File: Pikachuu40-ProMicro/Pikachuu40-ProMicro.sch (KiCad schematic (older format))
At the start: 93 parts, among them K1 KEYSW, K10 KEYSW, K11 KEYSW, K12 KEYSW, K13 KEYSW, K14 KEYSW, K15 KEYSW, K16 KEYSW, K17 KEYSW, K18 KEYSW, K19 KEYSW, K2 KEYSW, K20 KEYSW, K21 KEYSW, K22 KEYSW, K23 KEYSW, K24 KEYSW, K25 KEYSW, K26 KEYSW, K27 KEYSW, K28 KEYSW, K29 KEYSW, K3 KEYSW, K30 KEYSW, K31 KEYSW, K32 KEYSW, K33 KEYSW, K34 KEYSW, K35 KEYSW, K36 KEYSW, K37 KEYSW, K38 KEYSW, K39 KEYSW, K4 KEYSW, K40 KEYSW, K41 KEYSW, K42 KEYSW, K43 KEYSW, K44 KEYSW, K45 KEYSW, K5 KEYSW, K6 KEYSW, K7 KEYSW, K8 KEYSW, K9 KEYSW, U1 ProMicro

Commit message: Schematic done again
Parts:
- K1, K10, K11, K12, K13, K14, K15, K16, K17, K18, K19, K2, K20, K21, K22, K23, K24, K25, K26, K27, K28, K29, K3, K30, K31, K32, K33, K34, K35, K36, K37, K38, K39, K4, K40, K41, K42, K43, K44, K45, K5, K6, K7, K8, K9, K?1: footprint Keebio-Parts:MX_LED -> Button_Switch_Keyboard:SW_Cherry_MX_1.00u_PCB

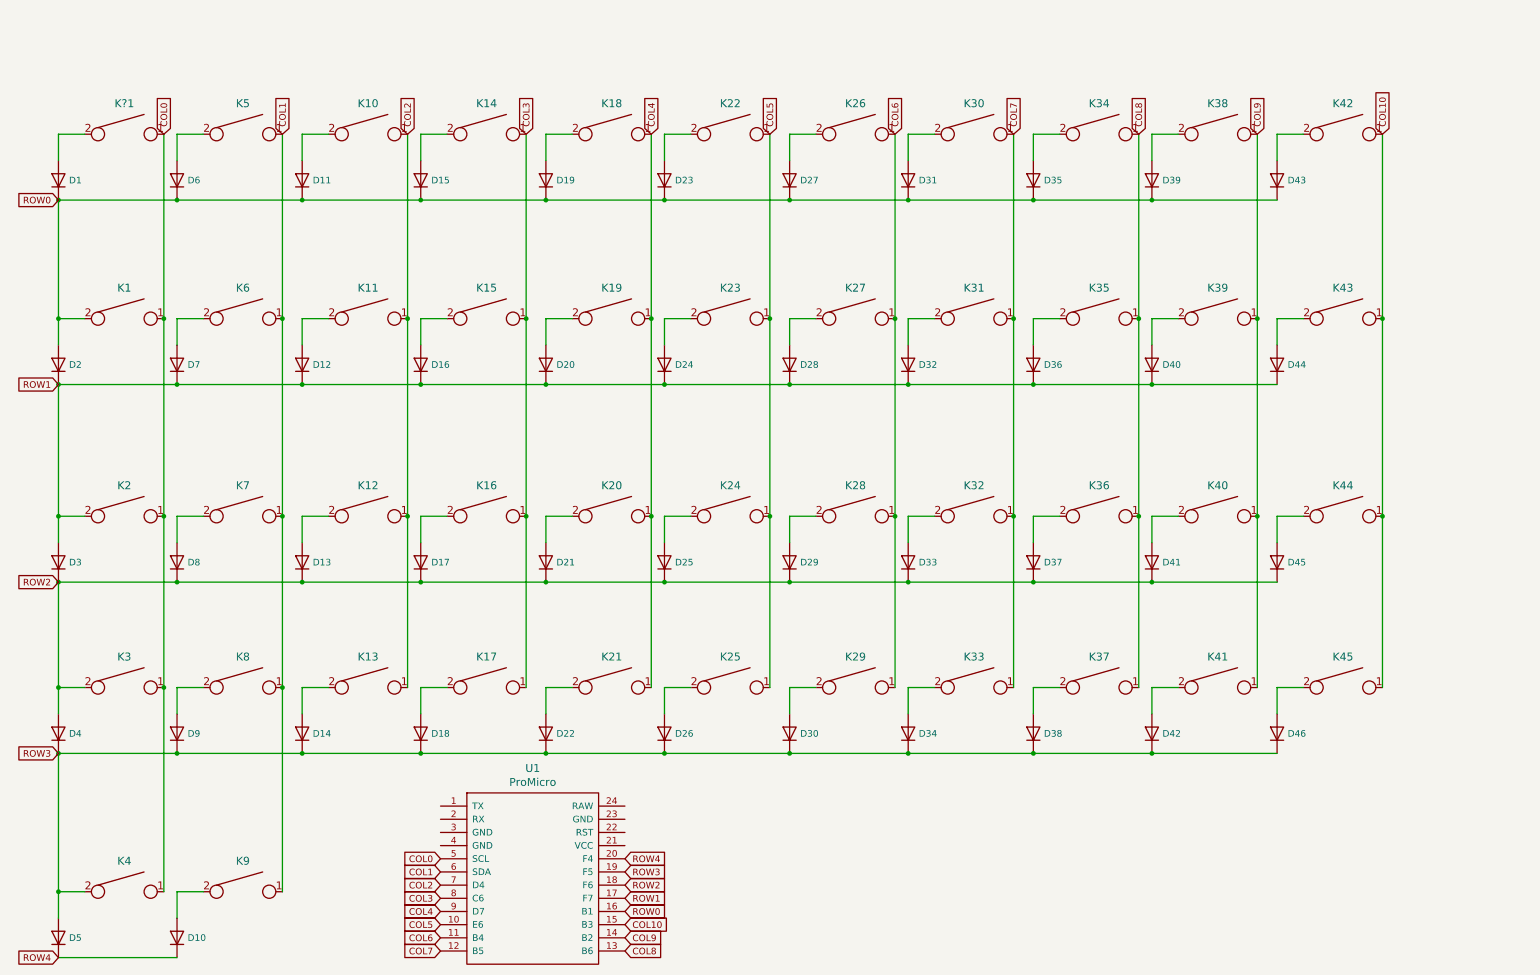
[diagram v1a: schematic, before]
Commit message: Rough Routing Done
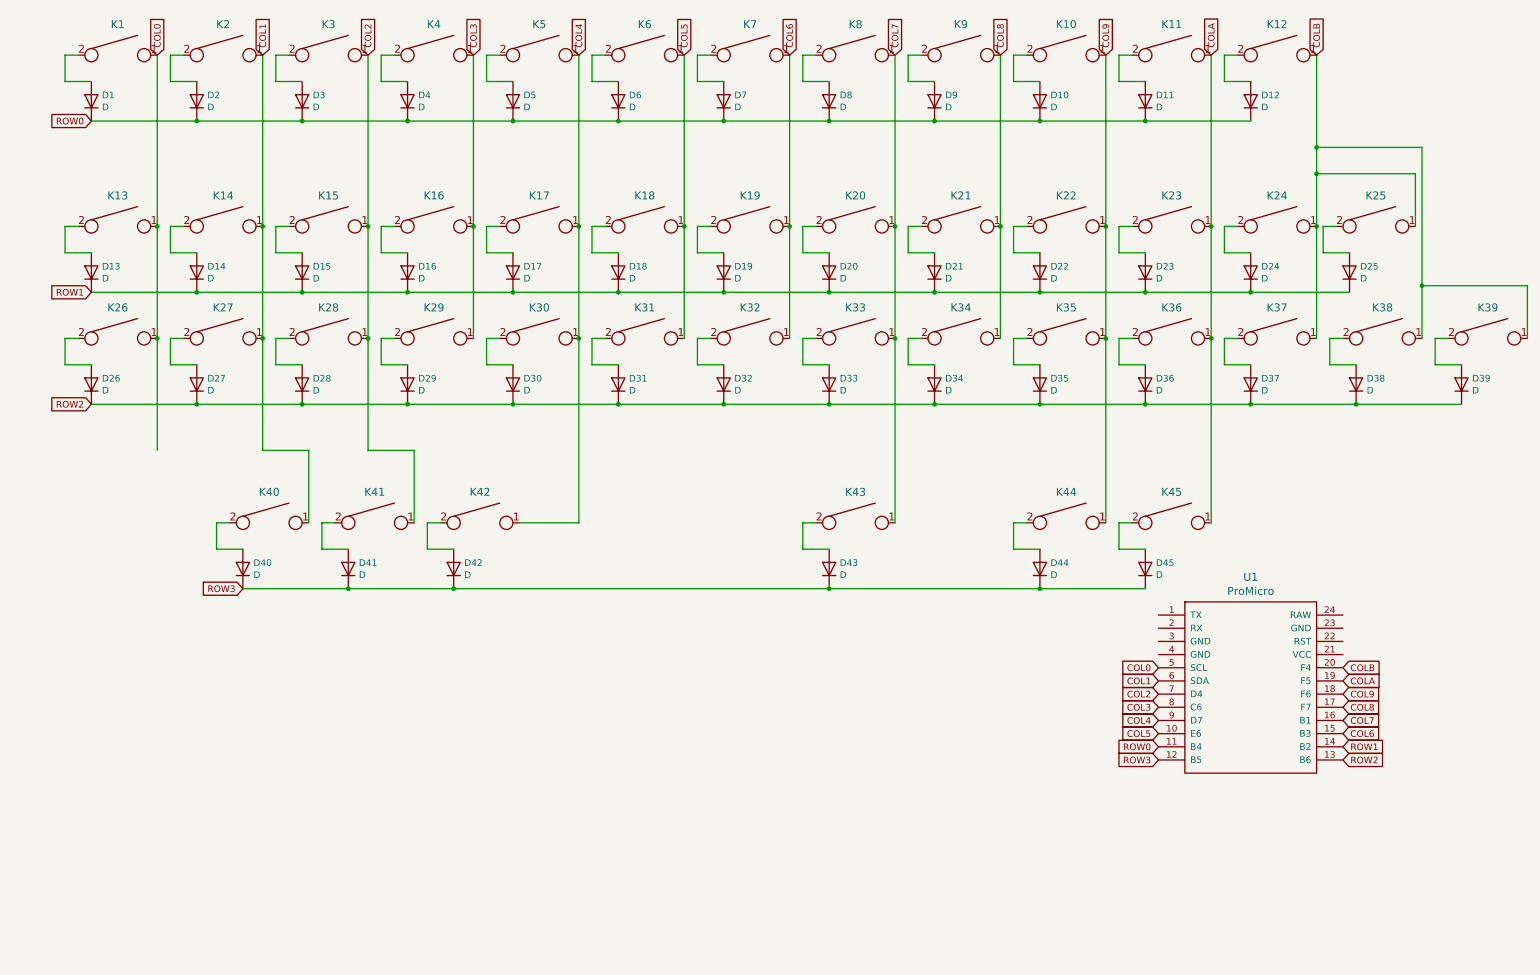
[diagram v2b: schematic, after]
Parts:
- removed D46: D, Keebio-Parts:Diode, symbol Device:D
- removed K?1: KEYSW, Button_Switch_Keyboard:SW_Cherry_MX_1.00u_PCB, symbol keyboard_parts:KEYSW
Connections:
- net COL0: now also K13.1, K26.1; no longer K2.1, K3.1, K4.1
- net COL1: now also K14.1, K2.1, K27.1, K40.1; no longer K5.1, K6.1, K7.1, K8.1, K9.1
- net COL2: now also K15.1, K28.1, K3.1, K41.1; no longer K10.1, K11.1, K12.1, K13.1
- net COL3: now also K29.1, K4.1; no longer K14.1, K15.1, K17.1
- net COL4: now also K17.1, K30.1, K42.1, K5.1; no longer K18.1, K19.1, K20.1, K21.1
- net COL5: now also K18.1, K31.1, K6.1; no longer K22.1, K23.1, K24.1, K25.1
- net COL6: now also K19.1, K32.1, K7.1, U1.15 (B3); no longer K26.1, K27.1, K28.1, K29.1, U1.11 (B4)
- net COL7: now also K20.1, K43.1, K8.1, U1.16 (B1); no longer K30.1, K31.1, K32.1, U1.12 (B5)
- net COL8: now also K21.1, K9.1, U1.17 (F7); no longer K35.1, K36.1, K37.1, U1.13 (B6)
- net COL9: now also K10.1, K22.1, K35.1, K44.1, U1.18 (F6); no longer K38.1, K39.1, K40.1, K41.1, U1.14 (B2)
- net ROW0: now also D10.1 (K), D12.1 (K), D2.1 (K), D3.1 (K), D4.1 (K), D5.1 (K), D7.1 (K), D8.1 (K), D9.1 (K), U1.11 (B4); no longer D15.1 (K), D19.1 (K), D2.2 (A), D23.1 (K), D27.1 (K), D31.1 (K), D35.1 (K), D39.1 (K), D43.1 (K), K1.2, U1.16 (B1)
- net ROW1: now also D13.1 (K), D14.1 (K), D15.1 (K), D17.1 (K), D18.1 (K), D19.1 (K), D21.1 (K), D22.1 (K), D23.1 (K), D25.1 (K), U1.14 (B2); no longer D12.1 (K), D2.1 (K), D28.1 (K), D3.2 (A), D32.1 (K), D36.1 (K), D40.1 (K), D44.1 (K), D7.1 (K), K2.2, U1.17 (F7)
- net ROW2: now also D26.1 (K), D27.1 (K), D28.1 (K), D30.1 (K), D31.1 (K), D32.1 (K), D34.1 (K), D35.1 (K), D36.1 (K), D38.1 (K), D39.1 (K), U1.13 (B6); no longer D13.1 (K), D17.1 (K), D21.1 (K), D25.1 (K), D3.1 (K), D4.2 (A), D41.1 (K), D45.1 (K), D8.1 (K), K3.2, U1.18 (F6)
- net ROW3: now also D40.1 (K), D41.1 (K), D43.1 (K), D44.1 (K), D45.1 (K), U1.12 (B5); no longer D14.1 (K), D18.1 (K), D22.1 (K), D26.1 (K), D30.1 (K), D34.1 (K), D38.1 (K), D4.1 (K), D5.2 (A), D9.1 (K), K4.2, U1.19 (F5)
- net at D1.2 (A): now also K1.2
- net at K5.2: now also D5.2 (A); no longer D6.2 (A)
- net at K10.2: now also D10.2 (A); no longer D11.2 (A)
- net at K14.2: now also D14.2 (A); no longer D15.2 (A)
- net at K18.2: now also D18.2 (A); no longer D19.2 (A)
- net at K22.2: now also D22.2 (A); no longer D23.2 (A)
- net at K26.2: now also D26.2 (A); no longer D27.2 (A)
- net at K30.2: now also D30.2 (A); no longer D31.2 (A)
- net at K34.2: now also D34.2 (A); no longer D35.2 (A)
- net at K38.2: now also D38.2 (A); no longer D39.2 (A)
- net at K42.2: now also D42.2 (A); no longer D43.2 (A)
- net at K9.2: now also D9.2 (A); no longer D10.2 (A)
- net at K6.2: now also D6.2 (A); no longer D7.2 (A)
- net at K11.2: now also D11.2 (A); no longer D12.2 (A)
- net at K15.2: now also D15.2 (A); no longer D16.2 (A)
- net at K19.2: now also D19.2 (A); no longer D20.2 (A)
- net at K23.2: now also D23.2 (A); no longer D24.2 (A)
- net at K27.2: now also D27.2 (A); no longer D28.2 (A)
- net at K31.2: now also D31.2 (A); no longer D32.2 (A)
- net at K35.2: now also D35.2 (A); no longer D36.2 (A)
- net at K39.2: now also D39.2 (A); no longer D40.2 (A)
- net at K43.2: now also D43.2 (A); no longer D44.2 (A)
- net at K7.2: now also D7.2 (A); no longer D8.2 (A)
- net at K12.2: now also D12.2 (A); no longer D13.2 (A)
- net at K16.2: now also D16.2 (A); no longer D17.2 (A)
- net at K20.2: now also D20.2 (A); no longer D21.2 (A)
- net at K24.2: now also D24.2 (A); no longer D25.2 (A)
- net at K28.2: now also D28.2 (A); no longer D29.2 (A)
- net at K32.2: now also D32.2 (A); no longer D33.2 (A)
- net at K36.2: now also D36.2 (A); no longer D37.2 (A)
- net at K40.2: now also D40.2 (A); no longer D41.2 (A)
- net at K44.2: now also D44.2 (A); no longer D45.2 (A)
- net at K8.2: now also D8.2 (A); no longer D9.2 (A)
- net at K13.2: now also D13.2 (A); no longer D14.2 (A)
- net at K17.2: now also D17.2 (A); no longer D18.2 (A)
- net at K21.2: now also D21.2 (A); no longer D22.2 (A)
- net at K25.2: now also D25.2 (A); no longer D26.2 (A)
- net at K29.2: now also D29.2 (A); no longer D30.2 (A)
- net at K33.2: now also D33.2 (A); no longer D34.2 (A)
- net at K37.2: now also D37.2 (A); no longer D38.2 (A)
- net at K41.2: now also D41.2 (A); no longer D42.2 (A)
- net at K45.2: now also D45.2 (A)
- removed net COL10: K42.1, K43.1, K44.1, K45.1, U1.15 (B3)
- removed net ROW4: D10.1 (K), D5.1 (K), U1.20 (F4)
- new net: D2.2 (A), K2.2
- new net: D3.2 (A), K3.2
- new net: D4.2 (A), K4.2
- new net COLA: K11.1, K23.1, K36.1, K45.1, U1.19 (F5)
- new net COLB: K12.1, K24.1, K25.1, K37.1, K38.1, K39.1, U1.20 (F4)
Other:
- moved on the sheet: U1
